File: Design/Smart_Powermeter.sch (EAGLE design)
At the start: 66 parts, among them IC1 AMS1117-3.3, IC3 ESP32-S2-MINI-1-N4R2, J1 AUDIO_JACK_TRRSSMD_RA, J2 AUDIO_JACK_TRRSSMD_RA, J3 AUDIO_JACK_TRRSSMD_RA, J4 AUDIO_JACK_TRRSSMD_RA, J5 AUDIO_JACK_TRRSSMD_RA, J6 AUDIO_JACK_TRRSSMD_RA, J8 USB-C, Q1 IRLML0100

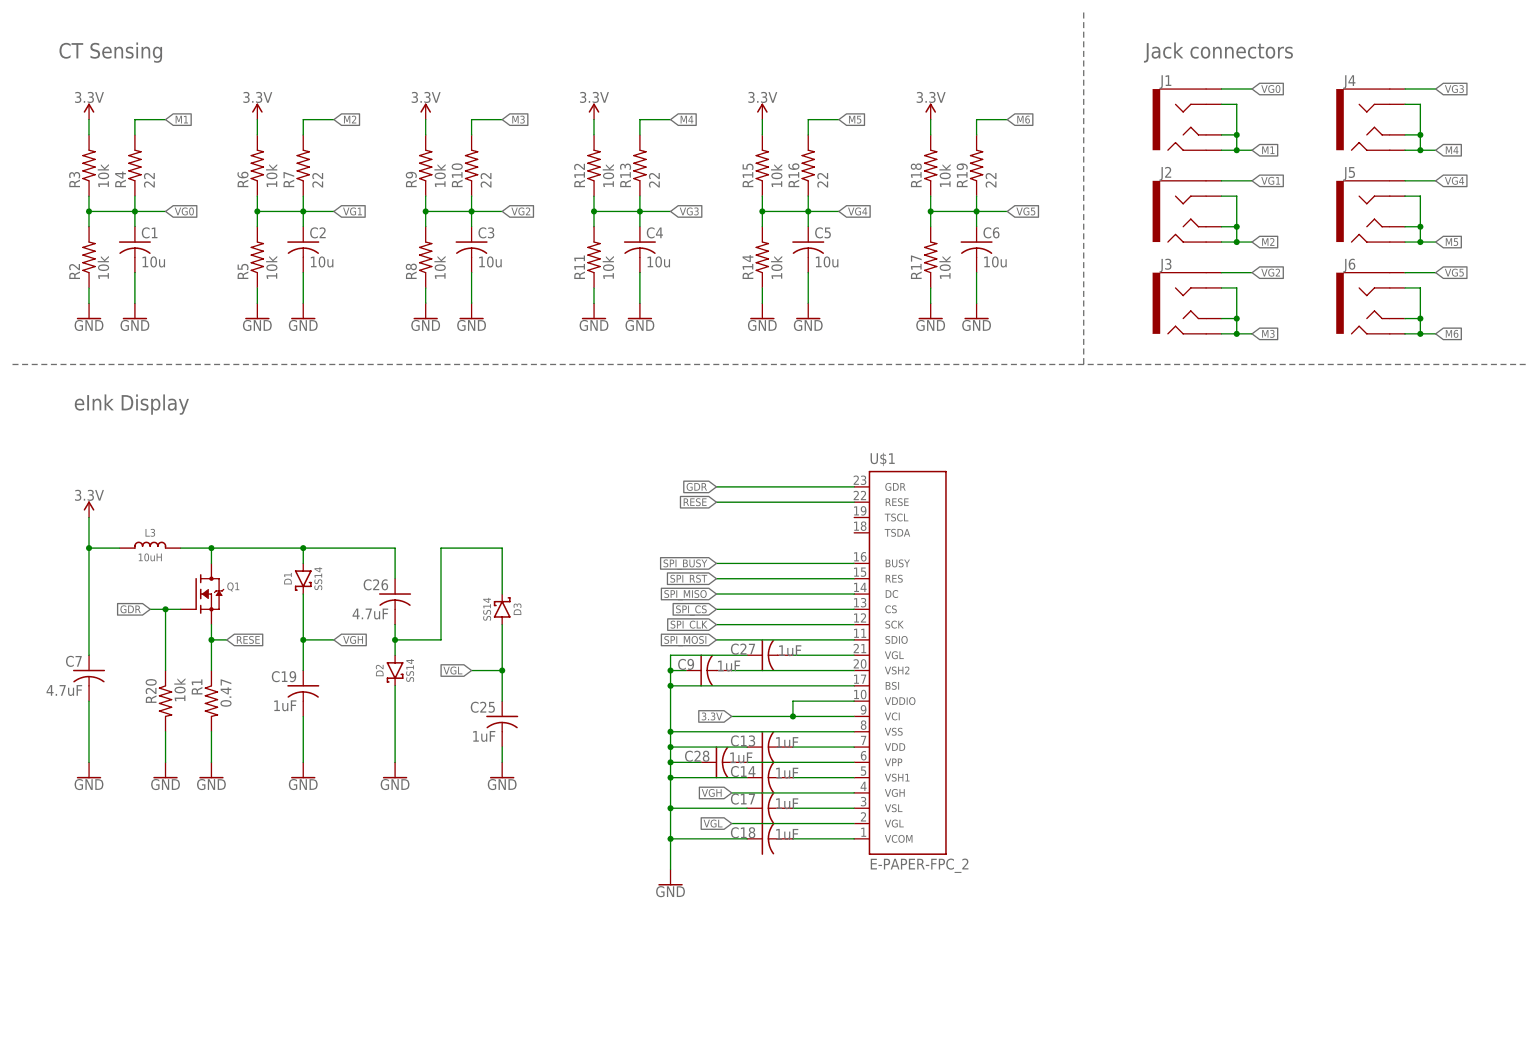
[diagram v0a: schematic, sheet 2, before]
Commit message: First draft for the Pro version
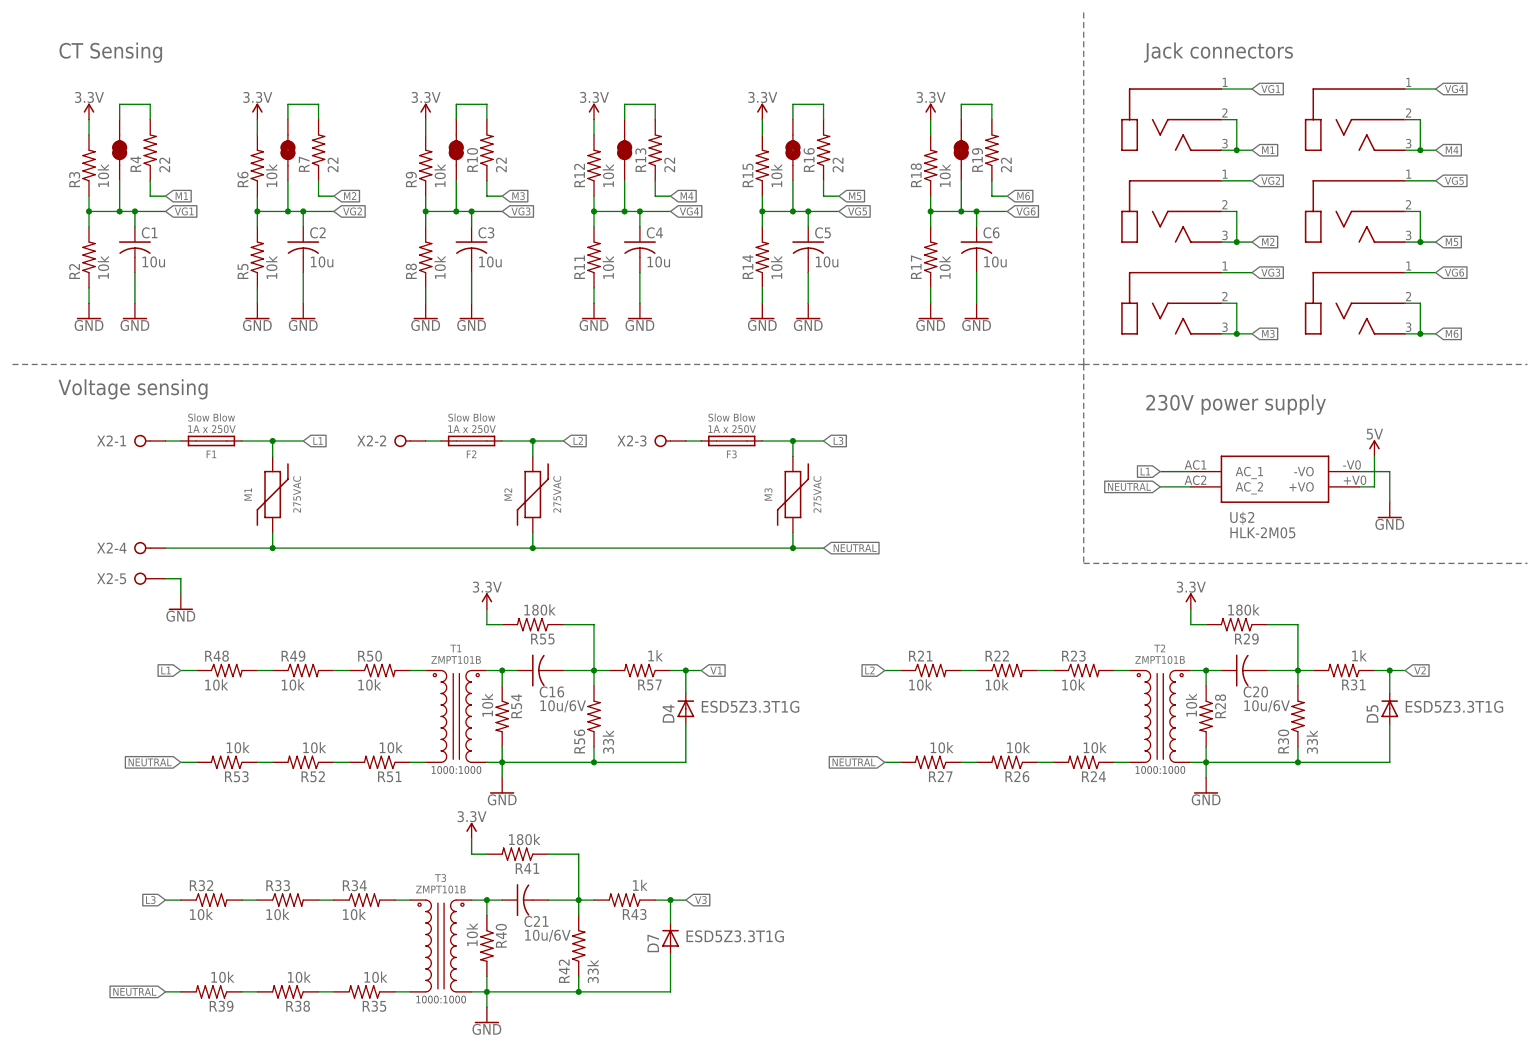
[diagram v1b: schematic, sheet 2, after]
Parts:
- removed X1: (no value), con-wago-508:W237-02P
- added C16, C20, C21: 10u/6V, rcl:C-USC0603
- added D4, D5, D7: ESD5Z3.3T1G, microbuilder:DIODESOD-523
- added F1, F2, F3: 1A x 250V, OpenEnergyMonitor:FUSE
- added JP1, JP2, JP3, JP4, JP5, JP6: JUMPER-SMT_2_NC_TRACE_NO-SILK, SparkFun-Jumpers:JUMPER-SMT_2_NC_TRACE_NO-SILK
- added M1, M2, M3: 275VAC, OpenEnergyMonitor:MOV_14MM_275VAC
- added R21, R22, R23, R24, R26, R27, R28, R32, R33, R34, R35, R38, R39, R40, R48, R49, R50, R51, R52, R53, R54: 10k, rcl:R-US_R0603
- added R29, R41, R55: 180k, rcl:R-US_R0603
- added R30, R42, R56: 33k, rcl:R-US_R0603
- added R31, R43, R57: 1k, rcl:R-US_R0603
- added T1, T2, T3: ZMPT101B, OpenEnergyMonitor:ZMPT101B
- added X2: (no value), con-wago-508:W237-05P
- J1, J2, J3, J4, J5, J6: value AUDIO_JACK_TRRSSMD_RA -> AUDIO_JACK_MONO_3.5_3P; device SparkFun-Connectors:AUDIO_JACK_TRRSSMD_RA -> SpaceDIY_connectors:AUDIO_JACK_MONO_3.5_3P
- R10, R13, R16, R19, R4, R7: device rcl:R-US_R1206 -> rcl:R-US_R0603
- U$2: LCSC (none) -> C209909
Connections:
- removed net VG0: C1.1, J1.EARTH, R2.2, R3.1, R4.1
- new net L1: F1.2, M1.2, R48.1, U$2.AC_1
- new net L2: F2.2, M2.2, R21.1
- new net L3: F3.2, M3.2, R32.1
- new net N$10: R23.2, T2.PRI_1
- new net N$18: C20.1, R28.1, T2.SEC_2
- new net N$19: C20.2, R29.1, R30.2, R31.2
- new net N$20: R32.2, R33.1
- new net N$21: R33.2, R34.1
- new net N$22: R35.1, T3.PRI_2
- new net N$23: R35.2, R38.1
- new net N$24: R38.2, R39.1
- new net N$25: R48.2, R49.1
- new net N$26: R34.2, T3.PRI_1
- new net N$27: C21.1, R40.1, T3.SEC_2
- new net N$28: C21.2, R41.1, R42.2, R43.2
- new net N$29: JP2.2, R7.2
- new net N$3: F2.1, X2-2.KL
- new net N$30: JP3.2, R10.2
- new net N$33: JP4.2, R13.2
- new net N$34: JP5.2, R16.2
- new net N$35: JP6.2, R19.2
- new net N$36: R49.2, R50.1
- new net N$37: R51.1, T1.PRI_2
- new net N$38: R51.2, R52.1
- new net N$39: R52.2, R53.1
- new net N$4: F3.1, X2-3.KL
- new net N$40: R50.2, T1.PRI_1
- new net N$41: C16.1, R54.1, T1.SEC_2
- new net N$44: C16.2, R55.1, R56.2, R57.2
- new net N$5: R21.2, R22.1
- new net N$6: R22.2, R23.1
- new net N$7: R24.1, T2.PRI_2
- new net N$8: R24.2, R26.1
- new net N$9: R26.2, R27.1
- new net NEUTRAL: M1.1, M2.1, M3.1, R27.2, R39.2, R53.2, U$2.AC_2, X2-4.KL
- new net V1: D4.C, R57.1
- new net V2: D5.C, R31.1
- new net V3: D7.C, R43.1
- new net VG6: C6.1, J6.1, JP6.1, R17.2, R18.1
- net 3.3V: now also R29.2, R41.2, R55.2
- net GND: now also D4.A, D5.A, D7.A, R28.2, R30.1, R40.2, R42.1, R54.2, R56.1, T1.SEC_1, T2.SEC_1, T3.SEC_1, X2-5.KL
- net M1: now also J1.2, J1.3, R4.1; no longer J1.RING1, J1.RING2, J1.TIP, R4.2
- net M2: now also J2.2, J2.3, R7.1; no longer J2.RING1, J2.RING2, J2.TIP, R7.2
- net M3: now also J3.2, J3.3, R10.1; no longer J3.RING1, J3.RING2, J3.TIP, R10.2
- net M4: now also J4.2, J4.3, R13.1; no longer J4.RING1, J4.RING2, J4.TIP, R13.2
- net M5: now also J5.2, J5.3, R16.1; no longer J5.RING1, J5.RING2, J5.TIP, R16.2
- net M6: now also J6.2, J6.3, R19.1; no longer J6.RING1, J6.RING2, J6.TIP, R19.2
- net N$1: now also JP1.2, R4.2; no longer U$2.AC_2, X1-2.KL
- net N$2: now also F1.1, X2-1.KL; no longer U$2.AC_1, X1-1.KL
- net VG1: now also C1.1, J1.1, JP1.1, R2.2, R3.1; no longer C2.1, J2.EARTH, R5.2, R6.1, R7.1
- net VG2: now also C2.1, J2.1, JP2.1, R5.2, R6.1; no longer C3.1, J3.EARTH, R10.1, R8.2, R9.1
- net VG3: now also C3.1, J3.1, JP3.1, R8.2, R9.1; no longer C4.1, J4.EARTH, R11.2, R12.1, R13.1
- net VG4: now also C4.1, J4.1, JP4.1, R11.2, R12.1; no longer C5.1, J5.EARTH, R14.2, R15.1, R16.1
- net VG5: now also C5.1, J5.1, JP5.1, R14.2, R15.1; no longer C6.1, J6.EARTH, R17.2, R18.1, R19.1
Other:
- note added: "Voltage sensing"
- moved on the sheet: C11, C12, IC3, J7, J9, R10, R13, R16, R19, R4, R7
